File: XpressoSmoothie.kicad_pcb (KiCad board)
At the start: 2 copper layers, 99.7 x 99.7 mm, 130 parts, among them J1 HEADER_4, J10 HEADER_3X2, J11 Pwr_in, J12 HEADER_4, J13 HEADER_4X2, J14 HEADER_3X2, J15 HEADER_4, J16 HEADER_4, J17 HEADER_4, J172 HEADER_2, J18 HEADER_4, J19 HEADER_2, J2 HEADER_4, J20 HEADER_2, J21 HEADER_2, J22 HEADER_2, J23 HEADER_4, J232 HEADER_2, J24 HEADER_4, J25 HEADER_4, J252 HEADER_2, J26 USB, J27 HEADER_4, J28 MICROSD-MOLEX, J3 HEADER_3, J4 HEADER_3X2, J5 HEADER_3X2, J6 LPCXPRESSO_GENERIC_HEADER, J7 HEADER_4, J8 HEADER_4, J9 HEADER_3X2, M1 LOGO_OSHW, M2 LOGO_OSHW, Q1 IRLB 8743, Q2 IRLB 8743, Q3 IRLB 8743, Q4 IRLB 8743, SW1 SW_PUSH, SW2 SW_PUSH, U1 POLOLU_A4988, U10 TC4422A, U11 TC4422A, U12 LM1117-3.3, U2 POLOLU_A4988, U3 POLOLU_A4988, U4 POLOLU_A4988, U5 POLOLU_A4988, U7 LM7809CT, U8 TC4422A, U9 TC4422A

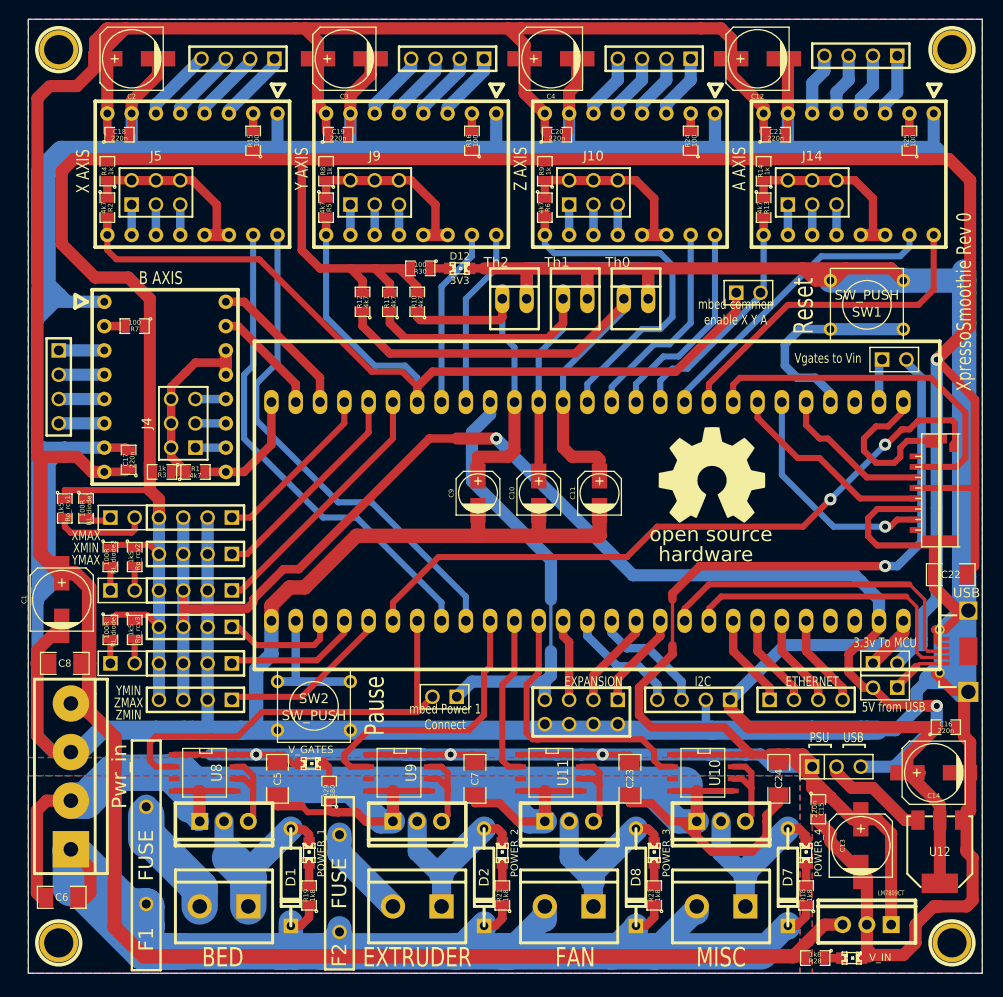
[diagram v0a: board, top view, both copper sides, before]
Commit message: fillzone
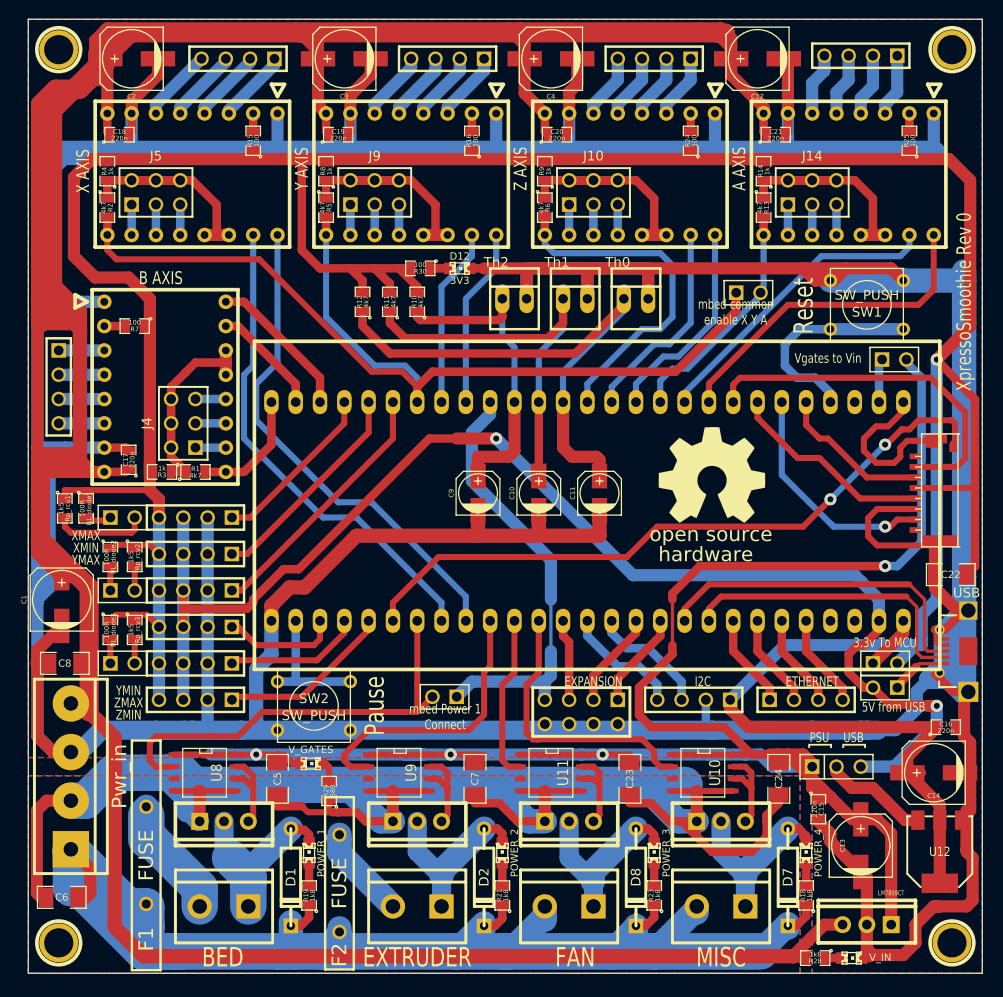
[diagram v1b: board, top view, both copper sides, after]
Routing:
- net Vin_rmot: track 317.8 -> 512.5 mm
- net +3.3VP: track 376.3 -> 374.1 mm
